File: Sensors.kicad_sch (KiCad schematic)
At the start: 22 parts, among them U3 INA226, U6 AS333

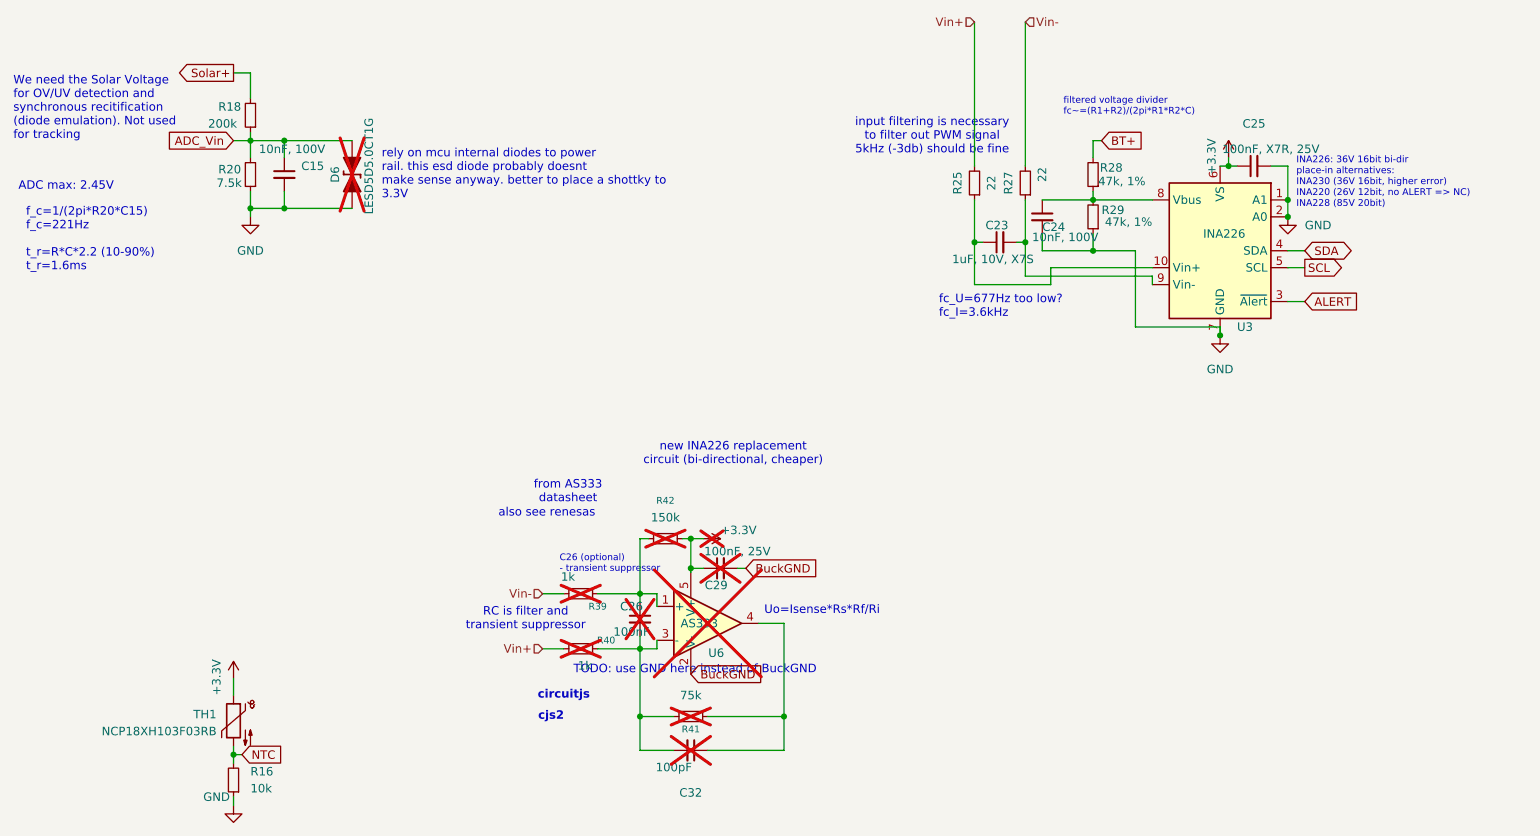
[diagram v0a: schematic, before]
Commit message: snap
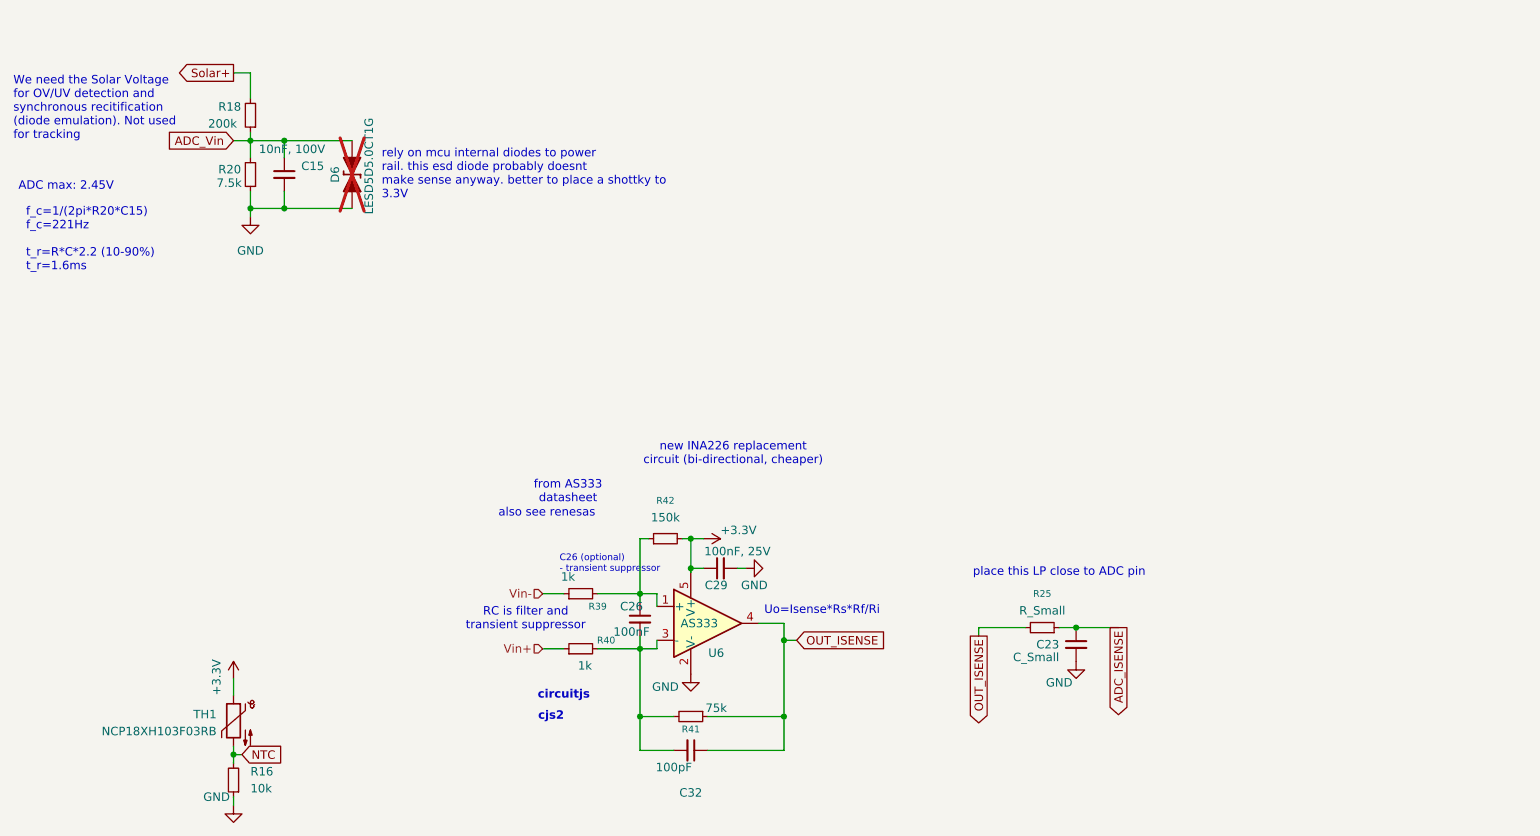
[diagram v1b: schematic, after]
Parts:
- removed C24: 10nF, 100V, Capacitor_SMD:C_0805_2012Metric, symbol Device:C_Small
- removed C25: 100nF, X7R, 25V, Capacitor_SMD:C_0805_2012Metric, symbol Device:C_Small
- removed R27: 22, Resistor_SMD:R_0805_2012Metric, symbol Device:R_Small
- removed R28, R29: 47k, 1%, Resistor_SMD:R_0805_2012Metric, symbol Device:R_Small
- removed U3: INA226, Package_SO:VSSOP-10_3x3mm_P0.5mm, symbol Sensor_Energy:INA226
- C23: value 1uF, 10V, X7S -> C_Small; Desc CS_Filt -> (none); Digikey CL21B105KAFNNNE -> (none); MPN 1uF, 10V, X7S -> (none)
- C26, C29, C32, R39, R40, R41, R42, U6: now fitted
- R25: value 22 -> R_Small; footprint Resistor_SMD:R_0805_2012Metric -> Resistor_SMD:R_0805_2012Metric_Pad1.20x1.40mm_HandSolder; Desc CS_FILT -> (none); MPN 22 -> (none)
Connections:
- net BuckGND is gone; now on net GND: C29.2, U6.2 (V-)
- net GND: now also C23.2
- net Vin+: no longer R25.2
- net ADC_ISENSE: now reaches C23.1, R25.1
- net OUT_ISENSE: now reaches C32.1, R41.1, U6.4
- net OUT_ISENSE: now also R25.2
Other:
- note added: "place this LP close to ADC pin"
- note removed: "INA226: 36V 16bit bi-dir place-in alternatives: INA230 (36V 16bit, higher error) INA220 (26V 12bit, no ALERT => NC) INA228 (85V 20bit)"
- note removed: "TODO: use GND here instead of BuckGND"
- note removed: "fc_U=677Hz too low? fc_I=3.6kHz"
- note removed: "filtered voltage divider fc~=(R1+R2)/(2pi*R1*R2*C)"
- note removed: "input filtering is necessary to filter out PWM signal 5kHz (-3db) should be fine"
